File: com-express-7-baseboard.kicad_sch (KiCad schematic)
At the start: 0 parts

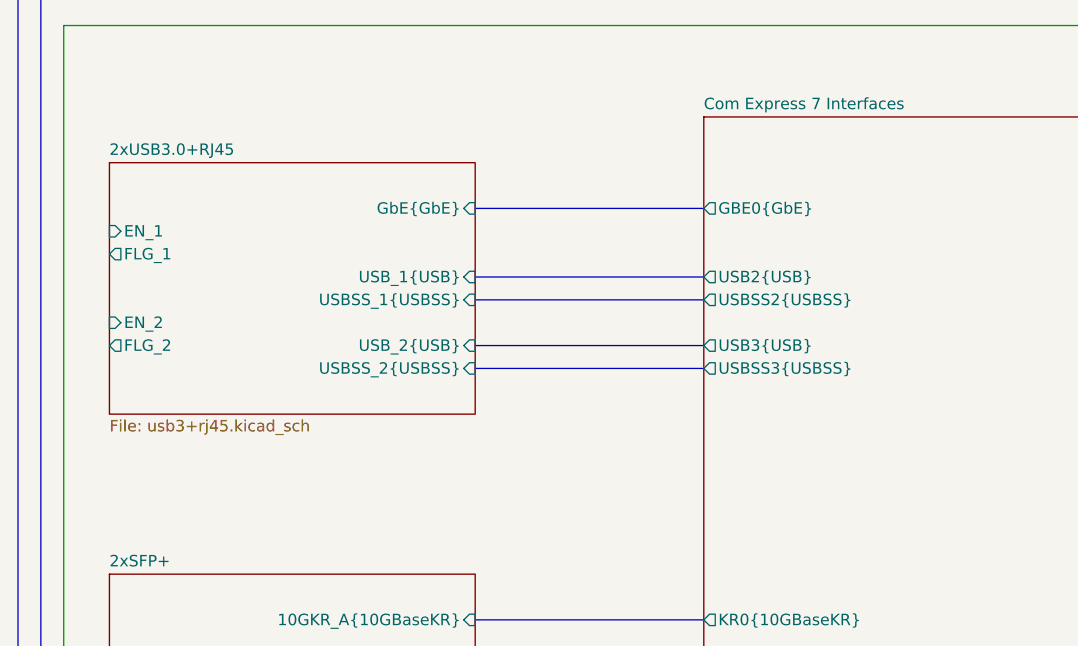
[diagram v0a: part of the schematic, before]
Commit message: [#57056] Connect GbE
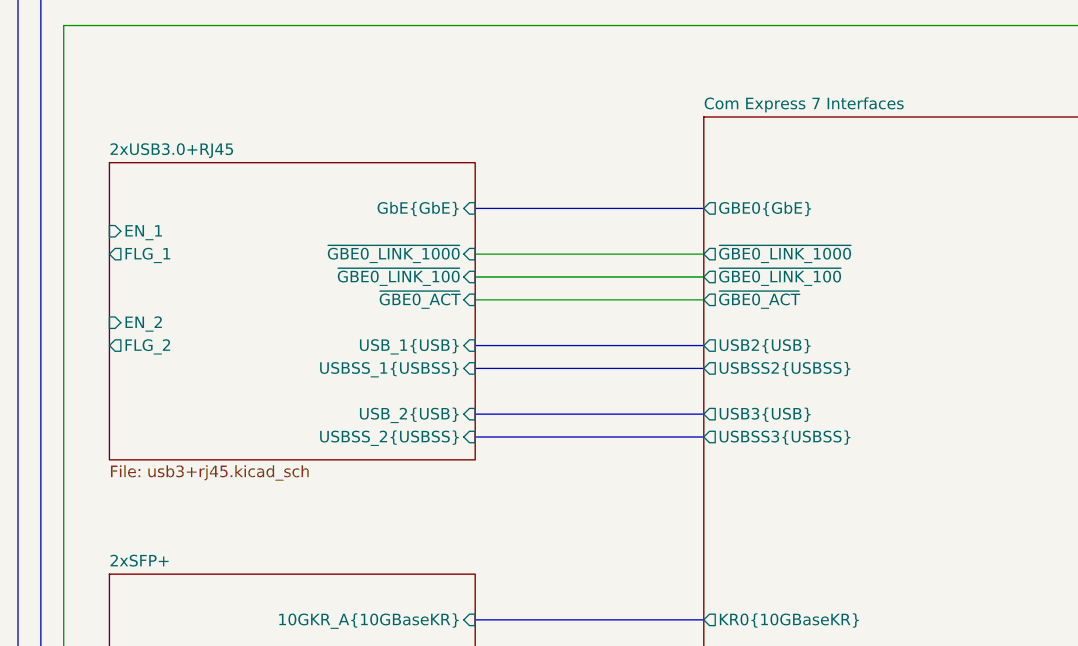
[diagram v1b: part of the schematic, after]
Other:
- sheet 2xUSB3.0+RJ45 ports: added ~{GBE0_ACT}, ~{GBE0_LINK_1000}, ~{GBE0_LINK_100}; removed none
- sheet Com Express 7 Interfaces ports: added ~{GBE0_ACT}, ~{GBE0_LINK_1000}, ~{GBE0_LINK_100}; removed none
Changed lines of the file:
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@@
     (stroke (width 0) (type default) (color 0 0 255 1))
   )
-  (bus (pts (xy 137.16 73.66) (xy 162.56 73.66))
+  (bus (pts (xy 137.16 81.28) (xy 162.56 81.28))
     (stroke (width 0) (type default) (color 0 255 255 1))
   )
@@
     (stroke (width 0) (type default) (color 255 0 0 1))
   )
+  (wire (pts (xy 137.16 73.66) (xy 162.56 73.66))
+    (stroke (width 0) (type default))
+  )
   (bus (pts (xy 96.52 152.4) (xy 86.36 152.4))
     (stroke (width 0) (type default))
@@
     (stroke (width 0) (type default))
   )
-  (bus (pts (xy 137.16 71.12) (xy 162.56 71.12))
+  (bus (pts (xy 137.16 78.74) (xy 162.56 78.74))
     (stroke (width 0) (type default) (color 0 0 255 1))
   )
@@
     (stroke (width 0) (type default))
   )
-  (bus (pts (xy 137.16 78.74) (xy 162.56 78.74))
+  (bus (pts (xy 137.16 86.36) (xy 162.56 86.36))
     (stroke (width 0) (type default) (color 0 0 255 1))
   )
@@
     (stroke (width 0) (type default))
   )
-  (bus (pts (xy 137.16 81.28) (xy 162.56 81.28))
+  (bus (pts (xy 137.16 88.9) (xy 162.56 88.9))
     (stroke (width 0) (type default) (color 0 255 255 1))
   )
@@
     (stroke (width 0) (type default))
   )
+  (wire (pts (xy 137.16 68.58) (xy 162.56 68.58))
+    (stroke (width 0) (type default))
+  )
   (bus (pts (xy 248.92 180.34) (xy 259.08 180.34))
     (stroke (width 0) (type default) (color 255 153 0 1))
@@
     (stroke (width 0) (type default))
   )
+  (wire (pts (xy 137.16 71.12) (xy 162.56 71.12))
+    (stroke (width 0) (type default))
+  )
   (wire (pts (xy 325.12 66.04) (xy 325.12 35.56))
     (stroke (width 0) (type default))
@@
       (effects (font (size 1.27 1.27)) (justify right))
     )
-    (pin "USB3{USB}" output (at 162.56 78.74 180)
-      (effects (font (size 1.27 1.27)) (justify left))
-    )
-    (pin "USB2{USB}" output (at 162.56 71.12 180)
+    (pin "USB3{USB}" output (at 162.56 86.36 180)
+      (effects (font (size 1.27 1.27)) (justify left))
+    )
+    (pin "USB2{USB}" output (at 162.56 78.74 180)
       (effects (font (size 1.27 1.27)) (justify left))
     )
@@
       (effects (font (size 1.27 1.27)) (justify right))
     )
-    (pin "USBSS3{USBSS}" output (at 162.56 81.28 180)
-      (effects (font (size 1.27 1.27)) (justify left))
-    )
-    (pin "USBSS2{USBSS}" output (at 162.56 73.66 180)
+    (pin "USBSS3{USBSS}" output (at 162.56 88.9 180)
+      (effects (font (size 1.27 1.27)) (justify left))
+    )
+    (pin "USBSS2{USBSS}" output (at 162.56 81.28 180)
       (effects (font (size 1.27 1.27)) (justify left))
     )
@@
       (effects (font (size 1.27 1.27)) (justify right))
     )
+    (pin "~{GBE0_ACT}" output (at 162.56 73.66 180)
+      (effects (font (size 1.27 1.27)) (justify left))
+    )
+    (pin "~{GBE0_LINK_1000}" output (at 162.56 68.58 180)
+      (effects (font (size 1.27 1.27)) (justify left))
+    )
+    (pin "~{GBE0_LINK_100}" output (at 162.56 71.12 180)
+      (effects (font (size 1.27 1.27)) (justify left))
+    )
     (instances
       (project "com-express-7-baseboard"
@@
     )
   )
-  (sheet (at 96.52 58.42) (size 40.64 27.94) (fields_autoplaced)
+  (sheet (at 96.52 58.42) (size 40.64 33.02) (fields_autoplaced)
     (stroke (width 0.1524) (type solid))
     (fill (color 0 0 0 0.0000))
@@
       (effects (font (size 1.27 1.27)) (justify left bottom))
     )
-    (property "Sheetfile" "usb3+rj45.kicad_sch" (at 96.52 86.9446 0)
+    (property "Sheetfile" "usb3+rj45.kicad_sch" (at 96.52 92.0246 0)
       (effects (font (size 1.27 1.27)) (justify left top))
     )
@@
       (effects (font (size 1.27 1.27)) (justify left))
     )
-    (pin "USB_1{USB}" input (at 137.16 71.12 0)
-      (effects (font (size 1.27 1.27)) (justify right))
-    )
-    (pin "USBSS_1{USBSS}" input (at 137.16 73.66 0)
-      (effects (font (size 1.27 1.27)) (justify right))
-    )
-    (pin "USB_2{USB}" input (at 137.16 78.74 0)
-      (effects (font (size 1.27 1.27)) (justify right))
-    )
-    (pin "USBSS_2{USBSS}" input (at 137.16 81.28 0)
+    (pin "USB_1{USB}" input (at 137.16 78.74 0)
+      (effects (font (size 1.27 1.27)) (justify right))
+    )
+    (pin "USBSS_1{USBSS}" input (at 137.16 81.28 0)
+      (effects (font (size 1.27 1.27)) (justify right))
+    )
+    (pin "USB_2{USB}" input (at 137.16 86.36 0)
+      (effects (font (size 1.27 1.27)) (justify right))
+    )
+    (pin "USBSS_2{USBSS}" input (at 137.16 88.9 0)
       (effects (font (size 1.27 1.27)) (justify right))
     )
@@
       (effects (font (size 1.27 1.27)) (justify left))
     )
-    (instances
+    (pin "~{GBE0_LINK_1000}" input (at 137.16 68.58 0)
+      (effects (font (size 1.27 1.27)) (justify right))
+    )
+    (pin "~{GBE0_ACT}" input (at 137.16 73.66 0)
+      (effects (font (size 1.27 1.27)) (justify right))
+    )
+    (pin "~{GBE0_LINK_100}" input (at 137.16 71.12 0)
+      (effects (font (size 1.27 1.27)) (justify right))
+    )
+    (instances
